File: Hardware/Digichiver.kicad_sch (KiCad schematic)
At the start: 3 parts, among them J2 USB4105-GF-A

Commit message: link footprints to symbols
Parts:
- R19, R20: footprint (none) -> Resistor_SMD:R_0402_1005Metric; MPN (none) -> RC0402FR-075K1L
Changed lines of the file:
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@@
 			)
 		)
-		(property "Footprint" ""
+		(property "Footprint" "Resistor_SMD:R_0402_1005Metric"
 			(at 139.446 110.236 90)
 			(hide yes)
@@
 			)
 		)
-		(property "Datasheet" ""
+		(property "Datasheet" "https://yageogroup.com/content/datasheet/asset/file/PYU-RC_GROUP_51_ROHS_L"
 			(at 139.7 109.22 0)
 			(hide yes)
@@
 		)
 		(property "KLC_S4.2_VREG_LX" ""
+			(at 139.7 109.22 90)
+			(hide yes)
+			(show_name no)
+			(do_not_autoplace no)
+			(effects
+				(font
+					(size 1.27 1.27)
+				)
+			)
+		)
+		(property "MPN" "RC0402FR-075K1L"
 			(at 139.7 109.22 90)
 			(hide yes)
@@
 			)
 		)
-		(property "Footprint" ""
+		(property "Footprint" "Resistor_SMD:R_0402_1005Metric"
 			(at 139.446 112.776 90)
 			(hide yes)
@@
 			)
 		)
-		(property "Datasheet" ""
+		(property "Datasheet" "https://yageogroup.com/content/datasheet/asset/file/PYU-RC_GROUP_51_ROHS_L"
 			(at 139.7 111.76 0)
 			(hide yes)
@@
 			(at 139.7 111.76 90)
 			(hide yes)
+			(show_name no)
+			(do_not_autoplace no)
+			(effects
+				(font
+					(size 1.27 1.27)
+				)
+			)
+		)
+		(property "MPN" "RC0402FR-075K1L"
+			(at 139.7 111.76 90)
+			(hide yes)

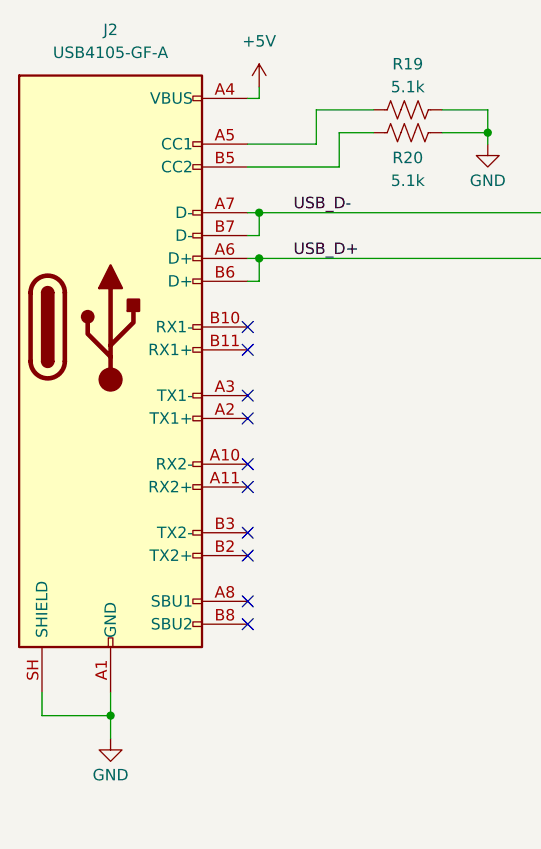
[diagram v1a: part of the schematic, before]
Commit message: layout complete
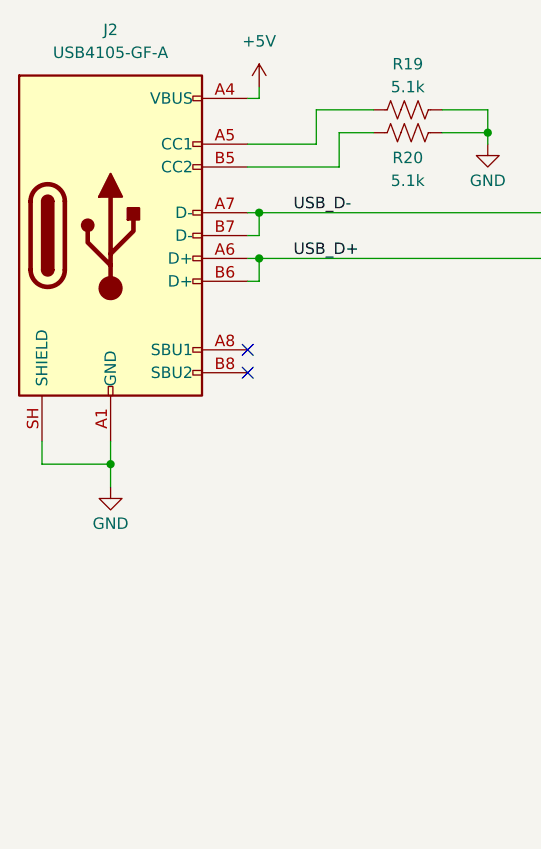
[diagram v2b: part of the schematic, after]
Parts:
- removed J2: USB4105-GF-A, Connector_USB:USB_C_Receptacle_GCT_USB4105-xx-A_16P_TopMnt_Horizontal, symbol Connector:USB_C_Receptacle
- added J2: USB4105-GF-A, Connector_USB:USB_C_Receptacle_GCT_USB4105-xx-A_16P_TopMnt_Horizontal, symbol Connector:USB_C_Receptacle_USB2.0_16P
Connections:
- net +5V: now also J2.A4 (VBUS), J2.A9 (VBUS), J2.B4 (VBUS), J2.B9 (VBUS)
- net GND: now also J2.A1 (GND), J2.A12 (GND), J2.B1 (GND), J2.B12 (GND), J2.SH (SHIELD)
- net USB_D+: now also J2.A6 (D+), J2.B6 (D+)
- net USB_D-: now also J2.A7 (D-), J2.B7 (D-)
- net at R19.2: now also J2.A5 (CC1)
- net at R20.2: now also J2.B5 (CC2)
- no-connect marks 10 -> 2
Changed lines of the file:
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@@
 	)
 	(junction
-		(at 106.68 176.53)
+		(at 106.68 148.59)
 		(diameter 0)
 		(color 0 0 0 0)
@@
 	)
 	(no_connect
-		(at 121.92 163.83)
-	)
-	(no_connect
-		(at 121.92 148.59)
-	)
-	(no_connect
-		(at 121.92 158.75)
-	)
-	(no_connect
-		(at 121.92 140.97)
-	)
-	(no_connect
-		(at 121.92 143.51)
+		(at 121.92 138.43)
 	)
 	(no_connect
 		(at 121.92 135.89)
 	)
-	(no_connect
-		(at 121.92 156.21)
-	)
-	(no_connect
-		(at 121.92 151.13)
-	)
-	(no_connect
-		(at 121.92 133.35)
-	)
-	(no_connect
-		(at 121.92 166.37)
-	)
 	(wire
 		(pts
@@
 	(wire
 		(pts
-			(xy 106.68 176.53) (xy 106.68 173.99)
+			(xy 106.68 148.59) (xy 106.68 146.05)
 		)
 		(stroke
@@
 	(wire
 		(pts
-			(xy 99.06 173.99) (xy 99.06 176.53)
+			(xy 99.06 146.05) (xy 99.06 148.59)
 		)
 		(stroke
@@
 	(wire
 		(pts
-			(xy 106.68 176.53) (xy 106.68 179.07)
+			(xy 106.68 148.59) (xy 106.68 151.13)
 		)
 		(stroke
@@
 	(wire
 		(pts
-			(xy 99.06 176.53) (xy 106.68 176.53)
+			(xy 99.06 148.59) (xy 106.68 148.59)
 		)
 		(stroke
@@
 				(path "/51de4045-d2a2-42d9-b145-319acd726bb6"
 					(reference "R19")
+					(unit 1)
+				)
+			)
+		)
+	)
+	(symbol
+		(lib_id "Connector:USB_C_Receptacle_USB2.0_16P")
+		(at 106.68 123.19 0)
+		(unit 1)
+		(body_style 1)
+		(exclude_from_sim no)
+		(in_bom yes)
+		(on_board yes)
+		(in_pos_files yes)
+		(dnp no)
+		(fields_autoplaced yes)
+		(property "Reference" "J2"
+			(at 106.68 100.33 0)
+			(show_name no)
+			(do_not_autoplace no)
+			(effects
+				(font
+					(size 1.27 1.27)
+				)
+			)
+		)
+		(property "Value" "USB4105-GF-A"
+			(at 106.68 102.87 0)
+			(show_name no)
+			(do_not_autoplace no)
+			(effects
+				(font
+					(size 1.27 1.27)
+				)
+			)
+		)
+		(property "Footprint" "Connector_USB:USB_C_Receptacle_GCT_USB4105-xx-A_16P_TopMnt_Horizontal"
+			(at 110.49 123.19 0)
+			(hide yes)
+			(show_name no)
+			(do_not_autoplace no)
+			(effects
+				(font
+					(size 1.27 1.27)
+				)
+			)
+		)
+		(property "Datasheet" "https://gct.co/files/drawings/usb4105.pdf"
+			(at 110.49 123.19 0)
+			(hide yes)
+			(show_name no)
+			(do_not_autoplace no)
+			(effects
+				(font
+					(size 1.27 1.27)
+				)
+			)
+		)
+		(property "Description" "USB 2.0-only 16P Type-C Receptacle connector"
+			(at 106.68 123.19 0)
+			(hide yes)
+			(show_name no)
+			(do_not_autoplace no)
+			(effects
+				(font
+					(size 1.27 1.27)
+				)
+			)
+		)
+		(property "MPN" "USB4105-GF-A"
+			(at 106.68 123.19 0)
+			(hide yes)
+			(show_name no)
+			(do_not_autoplace no)
+			(effects
+				(font
+					(size 1.27 1.27)
+				)
+			)
+		)
+		(pin "A4"
+		)
+		(pin "A8"
+		)
+		(pin "A12"
+		)
+		(pin "A1"
+		)
+		(pin "A5"
+		)
+		(pin "A6"
+		)
+		(pin "A7"
+		)
+		(pin "A9"
+		)
+		(pin "SH"
+		)
+		(pin "B8"
+		)
+		(pin "B7"
+		)
+		(pin "B1"
+		)
+		(pin "B12"
+		)
+		(pin "B4"
+		)
+		(pin "B6"
+		)
+		(pin "B9"
+		)
+		(pin "B5"
+		)
+		(instances
+			(project "Digichiver"
+				(path "/51de4045-d2a2-42d9-b145-319acd726bb6"
+					(reference "J2")
 					(unit 1)
 				)
@@
 	(symbol
 		(lib_id "power:GND")
-		(at 106.68 179.07 0)
+		(at 106.68 151.13 0)
 		(unit 1)
 		(body_style 1)
@@
 		(dnp no)
 		(property "Reference" "#PWR034"
-			(at 106.68 185.42 0)
+			(at 106.68 157.48 0)
 			(hide yes)
 			(show_name no)
@@
 		)
 		(property "Value" "GND"
-			(at 106.68 183.134 0)
+			(at 106.68 155.194 0)
 			(show_name no)
 			(do_not_autoplace no)
@@
 		)
 		(property "Footprint" ""
-			(at 106.68 179.07 0)
+			(at 106.68 151.13 0)
 			(hide yes)
 			(show_name no)
@@
 		)
 		(property "Datasheet" ""
-			(at 106.68 179.07 0)
+			(at 106.68 151.13 0)
 			(hide yes)
 			(show_name no)
@@
 		)
 		(property "Description" "Power symbol creates a global label with name \"GND\" , ground"
-			(at 106.68 179.07 0)
+			(at 106.68 151.13 0)
 			(hide yes)
 			(show_name no)
@@
 					(unit 1)
 				)
-			)
-		)
-	)
-	(symbol
-		(lib_id "Connector:USB_C_Receptacle")
-		(at 106.68 133.35 0)
-		(unit 1)
-		(body_style 1)
-		(exclude_from_sim no)
-		(in_bom yes)
-		(on_board yes)
-		(in_pos_files yes)
-		(dnp no)
-		(fields_autoplaced yes)
-		(property "Reference" "J2"
-			(at 106.68 100.33 0)
-			(show_name no)
-			(do_not_autoplace no)
-			(effects
-				(font
-					(size 1.27 1.27)
-				)
-			)
-		)
-		(property "Value" "USB4105-GF-A"
-			(at 106.68 102.87 0)
-			(show_name no)
-			(do_not_autoplace no)
-			(effects
-				(font
-					(size 1.27 1.27)
-				)
-			)
-		)
-		(property "Footprint" "Connector_USB:USB_C_Receptacle_GCT_USB4105-xx-A_16P_TopMnt_Horizontal"
-			(at 110.49 133.35 0)
-			(hide yes)
-			(show_name no)
-			(do_not_autoplace no)
-			(effects
-				(font
-					(size 1.27 1.27)
-				)
-			)
-		)
-		(property "Datasheet" "https://gct.co/files/drawings/usb4105.pdf"
-			(at 110.49 133.35 0)
-			(hide yes)
-			(show_name no)
-			(do_not_autoplace no)
-			(effects
-				(font
-					(size 1.27 1.27)
-				)
-			)
-		)
-		(property "Description" "USB Full-Featured Type-C Receptacle connector"
-			(at 106.68 133.35 0)
-			(hide yes)
-			(show_name no)
-			(do_not_autoplace no)
-			(effects
-				(font
-					(size 1.27 1.27)
-				)
-			)
-		)
-		(property "MPN" "USB4105-GF-A"
-			(at 106.68 133.35 0)
-			(hide yes)
-			(show_name no)
-			(do_not_autoplace no)
-			(effects
-				(font
-					(size 1.27 1.27)
-				)
-			)
-		)
-		(property "KLC_S4.2_DVDD" ""
-			(at 106.68 133.35 0)
-			(hide yes)
-			(show_name no)
-			(do_not_autoplace no)
-			(effects
-				(font
-					(size 1.27 1.27)
-				)
-			)
-		)
-		(property "KLC_S4.2_VREG_LX" ""
-			(at 106.68 133.35 0)
-			(hide yes)
-			(show_name no)
-			(do_not_autoplace no)
-			(effects
-				(font
-					(size 1.27 1.27)
-				)
-			)
-		)
-		(pin "B3"
-		)
-		(pin "A7"
-		)
-		(pin "A3"
-		)
-		(pin "A1"
-		)
-		(pin "A2"
-		)
-		(pin "A5"
-		)
-		(pin "A6"
-		)
-		(pin "A9"
-		)
-		(pin "A8"
-		)
-		(pin "A10"
-		)
-		(pin "A4"
-		)
-		(pin "A11"
-		)
-		(pin "A12"
-		)
-		(pin "B1"
-		)
-		(pin "B2"
-		)
-		(pin "B4"
-		)
-		(pin "B5"
-		)
-		(pin "B7"
-		)
-		(pin "B8"
-		)
-		(pin "B6"
-		)
-		(pin "B9"
-		)
-		(pin "B10"
-		)
-		(pin "B11"
-		)
-		(pin "B12"
-		)
-		(pin "SH"
-		)
-		(instances
-			(project "Digichiver"
-				(path "/51de4045-d2a2-42d9-b145-319acd726bb6"
-					(reference "J2")
-					(unit 1)
-				)

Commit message: generate outputs
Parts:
- J2: JLCPCB Part # (none) -> C3020560
- R19, R20: JLCPCB Part # (none) -> C105872
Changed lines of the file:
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@@
+			)
+		)
+		(property "JLCPCB Part #" "C105872"
+			(at 139.7 109.22 90)
+			(hide yes)
+			(show_name no)
+			(do_not_autoplace no)
+			(effects
+				(font
+					(size 1.27 1.27)
+				)
 			)
 		)
@@
 			)
 		)
+		(property "JLCPCB Part #" "C3020560"
+			(at 106.68 123.19 0)
+			(hide yes)
+			(show_name no)
+			(do_not_autoplace no)
+			(effects
+				(font
+					(size 1.27 1.27)
+				)
+			)
+		)
 		(pin "A4"
 		)
@@
 			(at 139.7 111.76 90)
 			(hide yes)
+			(show_name no)
+			(do_not_autoplace no)
+			(effects
+				(font
+					(size 1.27 1.27)
+				)
+			)
+		)
+		(property "JLCPCB Part #" "C105872"
+			(at 139.7 111.76 90)
+			(hide yes)
